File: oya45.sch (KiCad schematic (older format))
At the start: 108 parts, among them U1 ProMicro

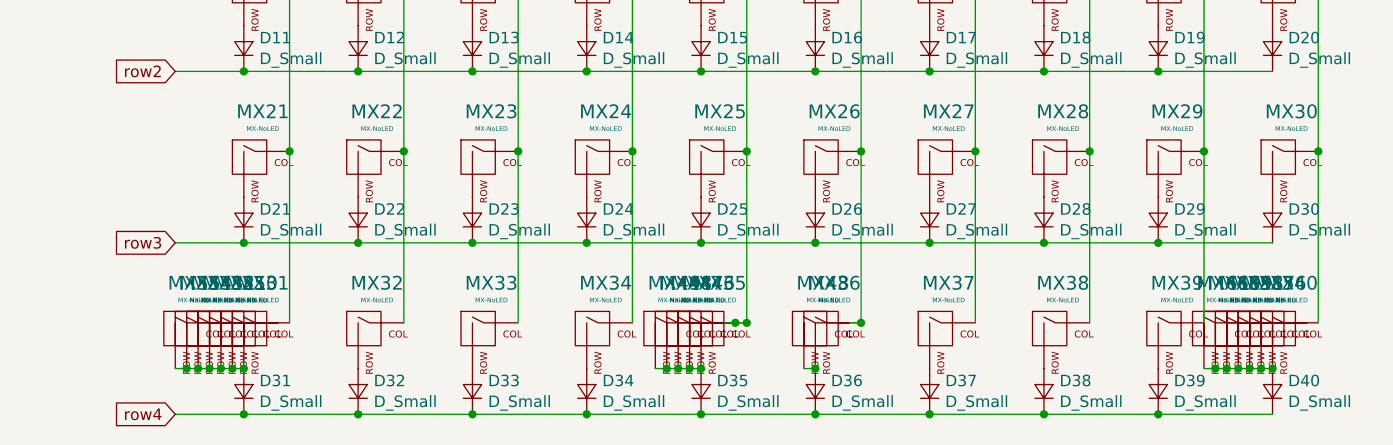
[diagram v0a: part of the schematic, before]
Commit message: fixed schematic
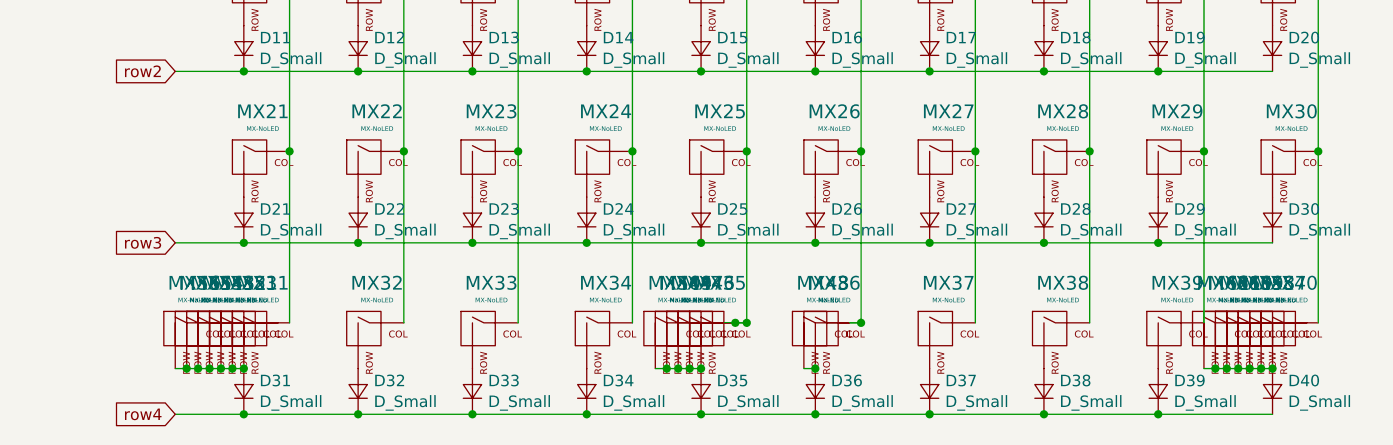
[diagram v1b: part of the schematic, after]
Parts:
- renumbered MX48 to MX49, MX49 to MX50, MX50 to MX51, MX51 to MX52, MX52 to MX53, MX53 to MX54, MX54 to MX55, MX55 to MX56, MX56 to MX57, MX57 to MX58, MX58 to MX59, MX59 to MX60, MX60 to MX61, MX61 to MX62
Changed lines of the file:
@@
 Connection ~ 7750 2550
 $Comp
-L MX_Alps_Hybrid:MX-NoLED MX50
-U 1 1 6130DEB4
-P 5550 4850
-F 0 "MX50" H 5583 5073 60  0000 C CNN
-F 1 "MX-NoLED" H 5583 4999 20  0000 C CNN
-F 2 "MX_Only:MXOnly-1U-NoLED" H 4925 4825 60  0001 C CNN
-F 3 "" H 4925 4825 60  0001 C CNN
-	1    5550 4850
-	1    0    0    -1
-$EndComp
-$Comp
-L MX_Alps_Hybrid:MX-NoLED MX51
-U 1 1 61310BF7
-P 5500 4850
-F 0 "MX51" H 5533 5073 60  0000 C CNN
-F 1 "MX-NoLED" H 5533 4999 20  0000 C CNN
-F 2 "MX_Only:MXOnly-1U-NoLED" H 4875 4825 60  0001 C CNN
-F 3 "" H 4875 4825 60  0001 C CNN
-	1    5500 4850
-	1    0    0    -1
-$EndComp
-$Comp
-L MX_Alps_Hybrid:MX-NoLED MX52
-U 1 1 6131191D
-P 5450 4850
-F 0 "MX52" H 5483 5073 60  0000 C CNN
-F 1 "MX-NoLED" H 5483 4999 20  0000 C CNN
-F 2 "MX_Only:MXOnly-1U-NoLED" H 4825 4825 60  0001 C CNN
-F 3 "" H 4825 4825 60  0001 C CNN
-	1    5450 4850
-	1    0    0    -1
-$EndComp
-$Comp
-L MX_Alps_Hybrid:MX-NoLED MX53
+L MX_Alps_Hybrid:MX-NoLED MX54
 U 1 1 61311AAE
 P 5400 4850
-F 0 "MX53" H 5433 5073 60  0000 C CNN
+F 0 "MX54" H 5433 5073 60  0000 C CNN
 F 1 "MX-NoLED" H 5433 4999 20  0000 C CNN
 F 2 "MX_Only:MXOnly-1U-NoLED" H 4775 4825 60  0001 C CNN
@@
 $EndComp
 $Comp
-L MX_Alps_Hybrid:MX-NoLED MX54
+L MX_Alps_Hybrid:MX-NoLED MX55
 U 1 1 61311CE4
 P 5350 4850
-F 0 "MX54" H 5383 5073 60  0000 C CNN
+F 0 "MX55" H 5383 5073 60  0000 C CNN
 F 1 "MX-NoLED" H 5383 4999 20  0000 C CNN
 F 2 "MX_Only:MXOnly-1U-NoLED" H 4725 4825 60  0001 C CNN
@@
 $EndComp
 $Comp
-L MX_Alps_Hybrid:MX-NoLED MX55
+L MX_Alps_Hybrid:MX-NoLED MX56
 U 1 1 61311E89
 P 5300 4850
-F 0 "MX55" H 5333 5073 60  0000 C CNN
+F 0 "MX56" H 5333 5073 60  0000 C CNN
 F 1 "MX-NoLED" H 5333 4999 20  0000 C CNN
 F 2 "MX_Only:MXOnly-1U-NoLED" H 4675 4825 60  0001 C CNN
@@
 $EndComp
 $Comp
-L MX_Alps_Hybrid:MX-NoLED MX56
+L MX_Alps_Hybrid:MX-NoLED MX57
 U 1 1 6131203D
 P 10050 4850
-F 0 "MX56" H 10083 5073 60  0000 C CNN
+F 0 "MX57" H 10083 5073 60  0000 C CNN
 F 1 "MX-NoLED" H 10083 4999 20  0000 C CNN
 F 2 "MX_Only:MXOnly-1U-NoLED" H 9425 4825 60  0001 C CNN
@@
 $EndComp
 $Comp
-L MX_Alps_Hybrid:MX-NoLED MX57
+L MX_Alps_Hybrid:MX-NoLED MX58
 U 1 1 6131231D
 P 10000 4850
-F 0 "MX57" H 10033 5073 60  0000 C CNN
+F 0 "MX58" H 10033 5073 60  0000 C CNN
 F 1 "MX-NoLED" H 10033 4999 20  0000 C CNN
 F 2 "MX_Only:MXOnly-1U-NoLED" H 9375 4825 60  0001 C CNN
@@
 $EndComp
 $Comp
-L MX_Alps_Hybrid:MX-NoLED MX58
+L MX_Alps_Hybrid:MX-NoLED MX59
 U 1 1 6131254E
 P 9950 4850
-F 0 "MX58" H 9983 5073 60  0000 C CNN
+F 0 "MX59" H 9983 5073 60  0000 C CNN
 F 1 "MX-NoLED" H 9983 4999 20  0000 C CNN
 F 2 "MX_Only:MXOnly-1U-NoLED" H 9325 4825 60  0001 C CNN
@@
 $EndComp
 $Comp
-L MX_Alps_Hybrid:MX-NoLED MX59
+L MX_Alps_Hybrid:MX-NoLED MX60
 U 1 1 6131279D
 P 9900 4850
-F 0 "MX59" H 9933 5073 60  0000 C CNN
+F 0 "MX60" H 9933 5073 60  0000 C CNN
 F 1 "MX-NoLED" H 9933 4999 20  0000 C CNN
 F 2 "MX_Only:MXOnly-1U-NoLED" H 9275 4825 60  0001 C CNN
@@
 $EndComp
 $Comp
-L MX_Alps_Hybrid:MX-NoLED MX60
+L MX_Alps_Hybrid:MX-NoLED MX61
 U 1 1 613129F6
 P 9850 4850
-F 0 "MX60" H 9883 5073 60  0000 C CNN
+F 0 "MX61" H 9883 5073 60  0000 C CNN
 F 1 "MX-NoLED" H 9883 4999 20  0000 C CNN
 F 2 "MX_Only:MXOnly-1U-NoLED" H 9225 4825 60  0001 C CNN
@@
 $EndComp
 $Comp
-L MX_Alps_Hybrid:MX-NoLED MX61
+L MX_Alps_Hybrid:MX-NoLED MX62
 U 1 1 61312BF5
 P 9800 4850
-F 0 "MX61" H 9833 5073 60  0000 C CNN
+F 0 "MX62" H 9833 5073 60  0000 C CNN
 F 1 "MX-NoLED" H 9833 4999 20  0000 C CNN
 F 2 "MX_Only:MXOnly-1U-NoLED" H 9175 4825 60  0001 C CNN
@@
 $EndComp
 $Comp
-L MX_Alps_Hybrid:MX-NoLED MX48
+L MX_Alps_Hybrid:MX-NoLED MX49
 U 1 1 61316CF3
 P 7450 4850
-F 0 "MX48" H 7483 5073 60  0000 C CNN
+F 0 "MX49" H 7483 5073 60  0000 C CNN
 F 1 "MX-NoLED" H 7483 4999 20  0000 C CNN
 F 2 "MX_Only:MXOnly-2U-ReversedStabilizers-NoLED" H 6825 4825 60  0001 C CNN
@@
 $EndComp
 $Comp
-L MX_Alps_Hybrid:MX-NoLED MX49
+L MX_Alps_Hybrid:MX-NoLED MX50
 U 1 1 61316F9C
 P 7400 4850
-F 0 "MX49" H 7433 5073 60  0000 C CNN
+F 0 "MX50" H 7433 5073 60  0000 C CNN
 F 1 "MX-NoLED" H 7433 4999 20  0000 C CNN
 F 2 "MX_Only:MXOnly-2U-ReversedStabilizers-NoLED" H 6775 4825 60  0001 C CNN
@@
 Wire Wire Line
 	7400 5000 7350 5000
-Connection ~ 5550 5000
 Wire Wire Line
 	5300 5000 5250 5000
@@
 	5400 5000 5350 5000
 Connection ~ 5400 5000
-Wire Wire Line
-	5450 5000 5400 5000
-Connection ~ 5450 5000
-Wire Wire Line
-	5550 5000 5500 5000
-Wire Wire Line
-	5500 5000 5450 5000
-Connection ~ 5500 5000
 Connection ~ 10050 5000
 Wire Wire Line
@@
 	10000 5000 9950 5000
 Connection ~ 10000 5000
+Connection ~ 5550 5000
+Connection ~ 5450 5000
+Wire Wire Line
+	5450 5000 5400 5000
+$Comp
+L MX_Alps_Hybrid:MX-NoLED MX52
+U 1 1 61310BF7
+P 5500 4850
+F 0 "MX52" H 5533 5073 60  0000 C CNN
+F 1 "MX-NoLED" H 5533 4999 20  0000 C CNN
+F 2 "MX_Only:MXOnly-1U-NoLED" H 4875 4825 60  0001 C CNN
+F 3 "" H 4875 4825 60  0001 C CNN
+	1    5500 4850
+	1    0    0    -1
+$EndComp
+Connection ~ 5500 5000
+Wire Wire Line
+	5500 5000 5450 5000
+Wire Wire Line
+	5550 5000 5500 5000
+$Comp
+L MX_Alps_Hybrid:MX-NoLED MX51
+U 1 1 6130DEB4
+P 5550 4850
+F 0 "MX51" H 5583 5073 60  0000 C CNN
+F 1 "MX-NoLED" H 5583 4999 20  0000 C CNN
+F 2 "MX_Only:MXOnly-1U-NoLED" H 4925 4825 60  0001 C CNN
+F 3 "" H 4925 4825 60  0001 C CNN
+	1    5550 4850
+	1    0    0    -1
+$EndComp
+$Comp
+L MX_Alps_Hybrid:MX-NoLED MX53
+U 1 1 6131191D
+P 5450 4850
+F 0 "MX53" H 5483 5073 60  0000 C CNN
+F 1 "MX-NoLED" H 5483 4999 20  0000 C CNN
+F 2 "MX_Only:MXOnly-1U-NoLED" H 4825 4825 60  0001 C CNN
+F 3 "" H 4825 4825 60  0001 C CNN
+	1    5450 4850
+	1    0    0    -1
+$EndComp
 $EndSCHEMATC

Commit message: finish schematics
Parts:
- MX49: footprint MX_Only:MXOnly-2U-ReversedStabilizers-NoLED -> MX_Only:MXOnly-6.25U-ReversedStabilizers-NoLED
- MX50: footprint MX_Only:MXOnly-2U-ReversedStabilizers-NoLED -> MX_Only:MXOnly-7U-ReversedStabilizers-NoLED
- MX51, MX52, MX53, MX57, MX58, MX59: footprint MX_Only:MXOnly-1U-NoLED -> MX_Only:MXOnly-1.25U-NoLED
- MX54, MX55, MX56, MX60, MX61, MX62: footprint MX_Only:MXOnly-1U-NoLED -> MX_Only:MXOnly-1.5U-NoLED
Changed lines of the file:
@@
 F 0 "MX54" H 5433 5073 60  0000 C CNN
 F 1 "MX-NoLED" H 5433 4999 20  0000 C CNN
-F 2 "MX_Only:MXOnly-1U-NoLED" H 4775 4825 60  0001 C CNN
+F 2 "MX_Only:MXOnly-1.5U-NoLED" H 4775 4825 60  0001 C CNN
 F 3 "" H 4775 4825 60  0001 C CNN
 	1    5400 4850
@@
 F 0 "MX55" H 5383 5073 60  0000 C CNN
 F 1 "MX-NoLED" H 5383 4999 20  0000 C CNN
-F 2 "MX_Only:MXOnly-1U-NoLED" H 4725 4825 60  0001 C CNN
+F 2 "MX_Only:MXOnly-1.5U-NoLED" H 4725 4825 60  0001 C CNN
 F 3 "" H 4725 4825 60  0001 C CNN
 	1    5350 4850
@@
 F 0 "MX56" H 5333 5073 60  0000 C CNN
 F 1 "MX-NoLED" H 5333 4999 20  0000 C CNN
-F 2 "MX_Only:MXOnly-1U-NoLED" H 4675 4825 60  0001 C CNN
+F 2 "MX_Only:MXOnly-1.5U-NoLED" H 4675 4825 60  0001 C CNN
 F 3 "" H 4675 4825 60  0001 C CNN
 	1    5300 4850
@@
 F 0 "MX57" H 10083 5073 60  0000 C CNN
 F 1 "MX-NoLED" H 10083 4999 20  0000 C CNN
-F 2 "MX_Only:MXOnly-1U-NoLED" H 9425 4825 60  0001 C CNN
+F 2 "MX_Only:MXOnly-1.25U-NoLED" H 9425 4825 60  0001 C CNN
 F 3 "" H 9425 4825 60  0001 C CNN
 	1    10050 4850
@@
 F 0 "MX58" H 10033 5073 60  0000 C CNN
 F 1 "MX-NoLED" H 10033 4999 20  0000 C CNN
-F 2 "MX_Only:MXOnly-1U-NoLED" H 9375 4825 60  0001 C CNN
+F 2 "MX_Only:MXOnly-1.25U-NoLED" H 9375 4825 60  0001 C CNN
 F 3 "" H 9375 4825 60  0001 C CNN
 	1    10000 4850
@@
 F 0 "MX59" H 9983 5073 60  0000 C CNN
 F 1 "MX-NoLED" H 9983 4999 20  0000 C CNN
-F 2 "MX_Only:MXOnly-1U-NoLED" H 9325 4825 60  0001 C CNN
+F 2 "MX_Only:MXOnly-1.25U-NoLED" H 9325 4825 60  0001 C CNN
 F 3 "" H 9325 4825 60  0001 C CNN
 	1    9950 4850
@@
 F 0 "MX60" H 9933 5073 60  0000 C CNN
 F 1 "MX-NoLED" H 9933 4999 20  0000 C CNN
-F 2 "MX_Only:MXOnly-1U-NoLED" H 9275 4825 60  0001 C CNN
+F 2 "MX_Only:MXOnly-1.5U-NoLED" H 9275 4825 60  0001 C CNN
 F 3 "" H 9275 4825 60  0001 C CNN
 	1    9900 4850
@@
 F 0 "MX61" H 9883 5073 60  0000 C CNN
 F 1 "MX-NoLED" H 9883 4999 20  0000 C CNN
-F 2 "MX_Only:MXOnly-1U-NoLED" H 9225 4825 60  0001 C CNN
+F 2 "MX_Only:MXOnly-1.5U-NoLED" H 9225 4825 60  0001 C CNN
 F 3 "" H 9225 4825 60  0001 C CNN
 	1    9850 4850
@@
 F 0 "MX62" H 9833 5073 60  0000 C CNN
 F 1 "MX-NoLED" H 9833 4999 20  0000 C CNN
-F 2 "MX_Only:MXOnly-1U-NoLED" H 9175 4825 60  0001 C CNN
+F 2 "MX_Only:MXOnly-1.5U-NoLED" H 9175 4825 60  0001 C CNN
 F 3 "" H 9175 4825 60  0001 C CNN
 	1    9800 4850
@@
 F 0 "MX49" H 7483 5073 60  0000 C CNN
 F 1 "MX-NoLED" H 7483 4999 20  0000 C CNN
-F 2 "MX_Only:MXOnly-2U-ReversedStabilizers-NoLED" H 6825 4825 60  0001 C CNN
+F 2 "MX_Only:MXOnly-6.25U-ReversedStabilizers-NoLED" H 6825 4825 60  0001 C CNN
 F 3 "" H 6825 4825 60  0001 C CNN
 	1    7450 4850
@@
 F 0 "MX50" H 7433 5073 60  0000 C CNN
 F 1 "MX-NoLED" H 7433 4999 20  0000 C CNN
-F 2 "MX_Only:MXOnly-2U-ReversedStabilizers-NoLED" H 6775 4825 60  0001 C CNN
+F 2 "MX_Only:MXOnly-7U-ReversedStabilizers-NoLED" H 6775 4825 60  0001 C CNN
 F 3 "" H 6775 4825 60  0001 C CNN
 	1    7400 4850
@@
 F 0 "MX52" H 5533 5073 60  0000 C CNN
 F 1 "MX-NoLED" H 5533 4999 20  0000 C CNN
-F 2 "MX_Only:MXOnly-1U-NoLED" H 4875 4825 60  0001 C CNN
+F 2 "MX_Only:MXOnly-1.25U-NoLED" H 4875 4825 60  0001 C CNN
 F 3 "" H 4875 4825 60  0001 C CNN
 	1    5500 4850
@@
 F 0 "MX51" H 5583 5073 60  0000 C CNN
 F 1 "MX-NoLED" H 5583 4999 20  0000 C CNN
-F 2 "MX_Only:MXOnly-1U-NoLED" H 4925 4825 60  0001 C CNN
+F 2 "MX_Only:MXOnly-1.25U-NoLED" H 4925 4825 60  0001 C CNN
 F 3 "" H 4925 4825 60  0001 C CNN
 	1    5550 4850
@@
 F 0 "MX53" H 5483 5073 60  0000 C CNN
 F 1 "MX-NoLED" H 5483 4999 20  0000 C CNN
-F 2 "MX_Only:MXOnly-1U-NoLED" H 4825 4825 60  0001 C CNN
+F 2 "MX_Only:MXOnly-1.25U-NoLED" H 4825 4825 60  0001 C CNN
 F 3 "" H 4825 4825 60  0001 C CNN
 	1    5450 4850
